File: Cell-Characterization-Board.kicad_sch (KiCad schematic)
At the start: 5 parts, among them IC2 INA4180A2IPWR, SW1 SW_Push, U1 ESP32-S3-WROOM-1

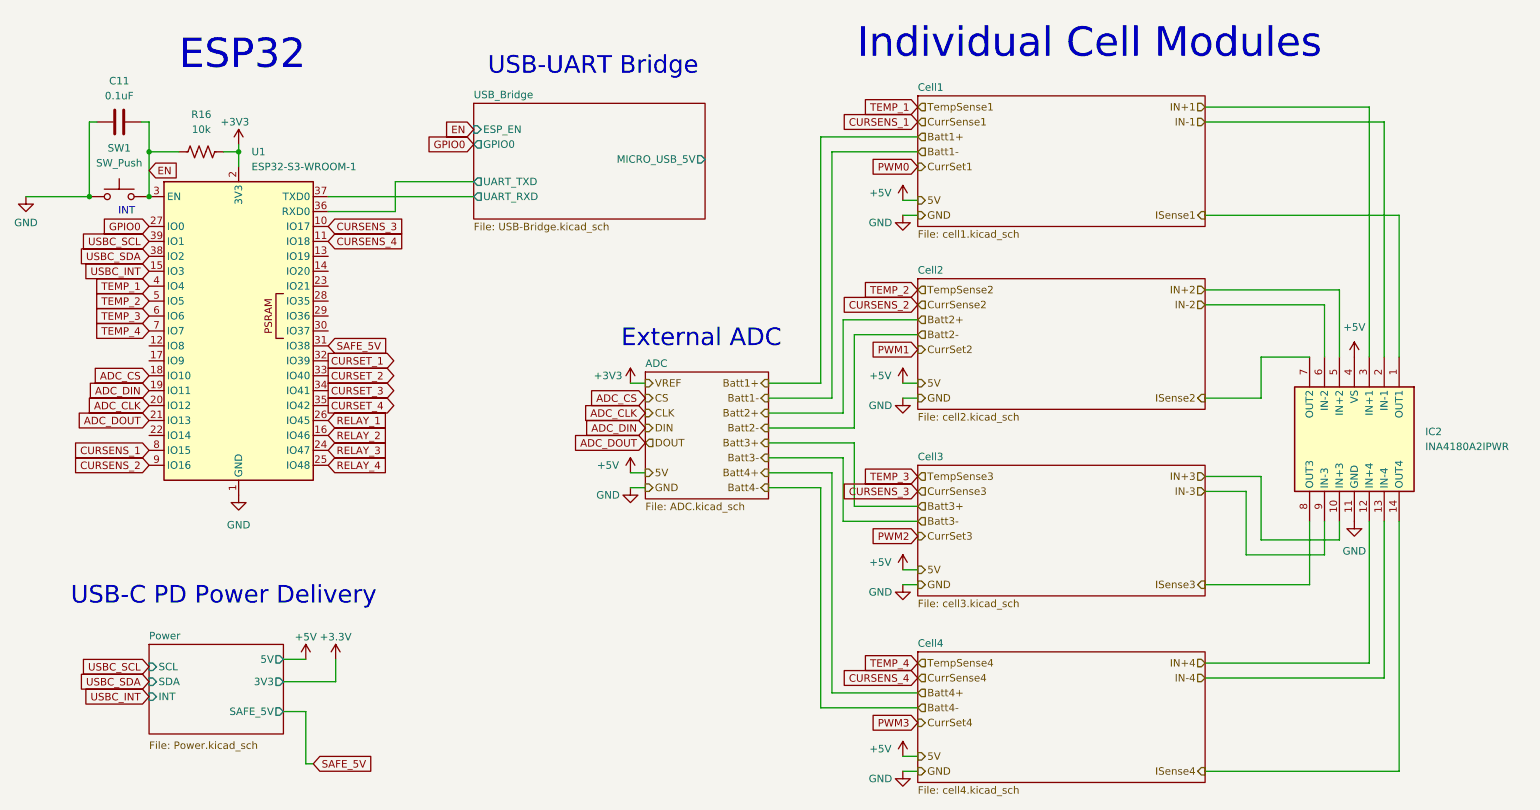
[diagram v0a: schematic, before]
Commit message: initial sch completed
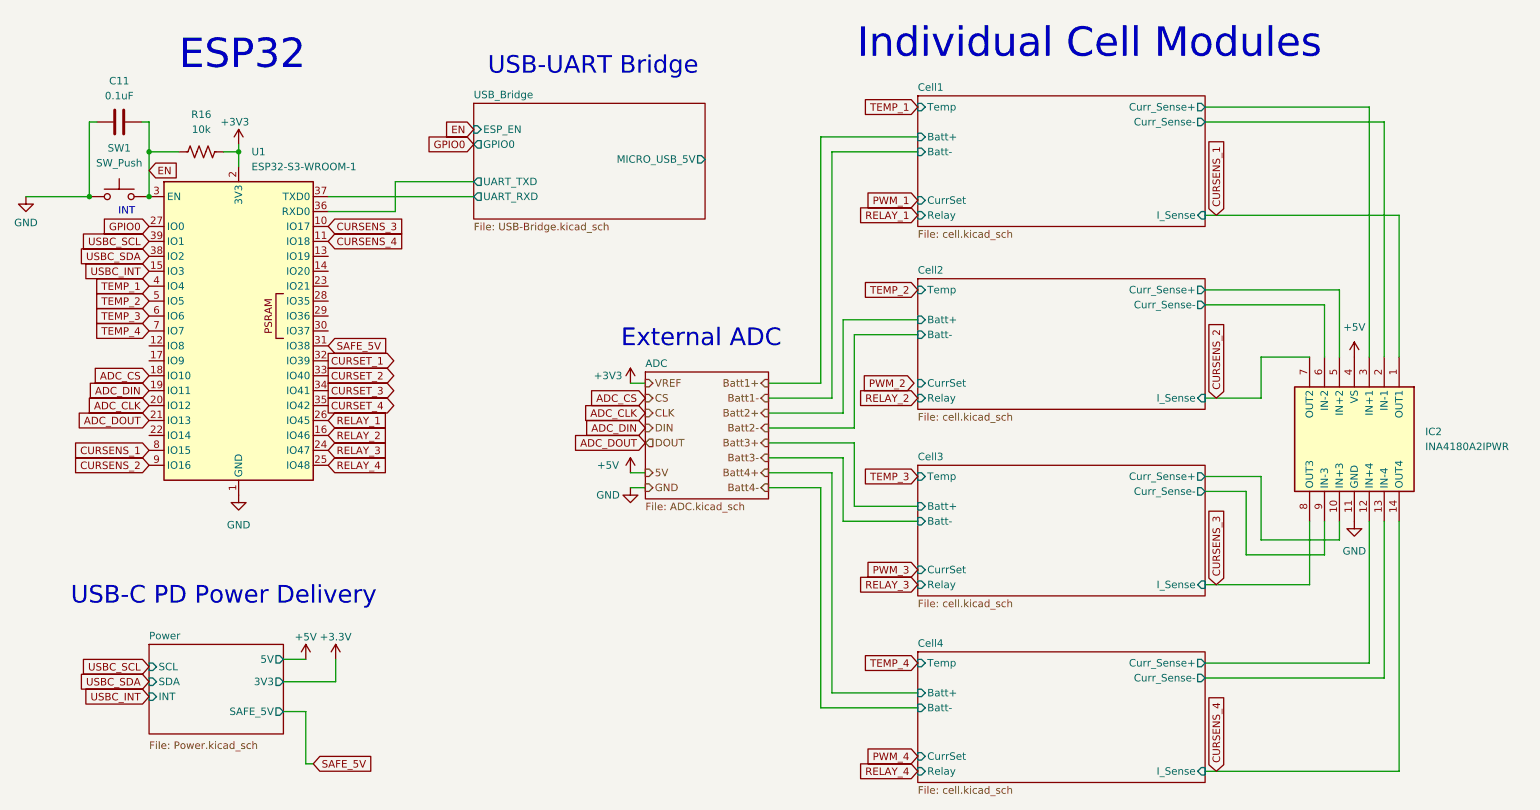
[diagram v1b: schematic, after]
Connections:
- net ISense1 is gone; now on net CURSENS_1: IC2.1 (OUT1)
- net ISense2 is gone; now on net CURSENS_2: IC2.7 (OUT2)
- net ISense3 is gone; now on net CURSENS_3: IC2.8 (OUT3)
- net ISense4 is gone; now on net CURSENS_4: IC2.14 (OUT4)
- net IN+1 renamed Cell1/Curr_Sense+
- net IN+2 renamed Cell2/Curr_Sense+
- net IN+3 renamed Cell3/Curr_Sense+
- net IN+4 renamed Cell4/Curr_Sense+
- net IN-1 renamed Cell1/Curr_Sense-
- net IN-2 renamed Cell2/Curr_Sense-
- net IN-3 renamed Cell3/Curr_Sense-
- net IN-4 renamed Cell4/Curr_Sense-
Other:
- sheet Cell1: file cell1.kicad_sch -> cell.kicad_sch
- sheet Cell1 ports: added Batt+, Batt-, CurrSet, Curr_Sense+, Curr_Sense-, I_Sense, Relay, Temp; removed none
- sheet Cell2: file cell2.kicad_sch -> cell.kicad_sch
- sheet Cell2 ports: added Batt+, Batt-, CurrSet, Curr_Sense+, Curr_Sense-, I_Sense, Relay, Temp; removed none
- sheet Cell3: file cell3.kicad_sch -> cell.kicad_sch
- sheet Cell3 ports: added Batt+, Batt-, CurrSet, Curr_Sense+, Curr_Sense-, I_Sense, Relay, Temp; removed none
- sheet Cell4: file cell4.kicad_sch -> cell.kicad_sch
- sheet Cell4 ports: added Batt+, Batt-, CurrSet, Curr_Sense+, Curr_Sense-, I_Sense, Relay, Temp; removed none
